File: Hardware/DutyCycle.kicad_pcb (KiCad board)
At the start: 2 copper layers, 40 x 20 mm, 39 parts, among them J1 LiPo, J2 USB, J4 MOT, Q1 AO3400A, Q2 AO3400A, Q3 AO3401A, SW1 SW_Push, U1 AT32F421KxU7, U3 ME6211C28M5, U5 TP4055

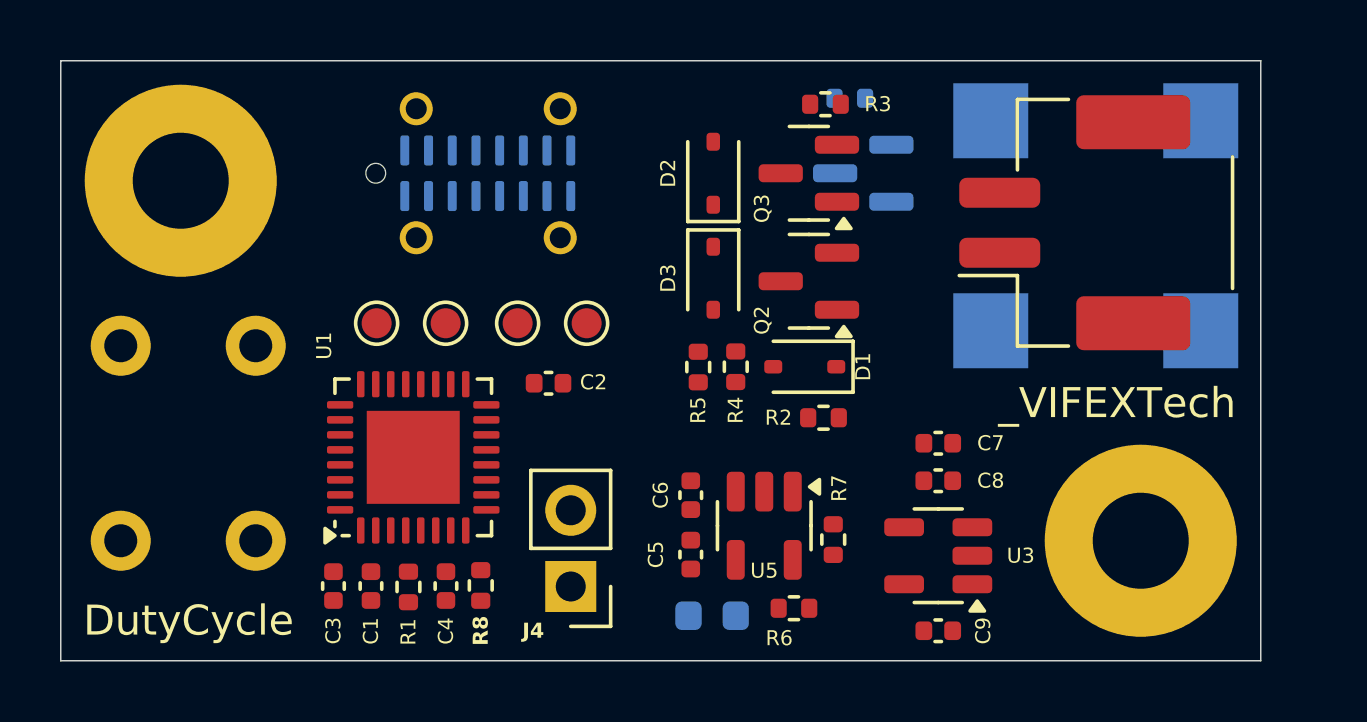
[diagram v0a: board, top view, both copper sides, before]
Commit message: feat(pcb): finish PCB layout
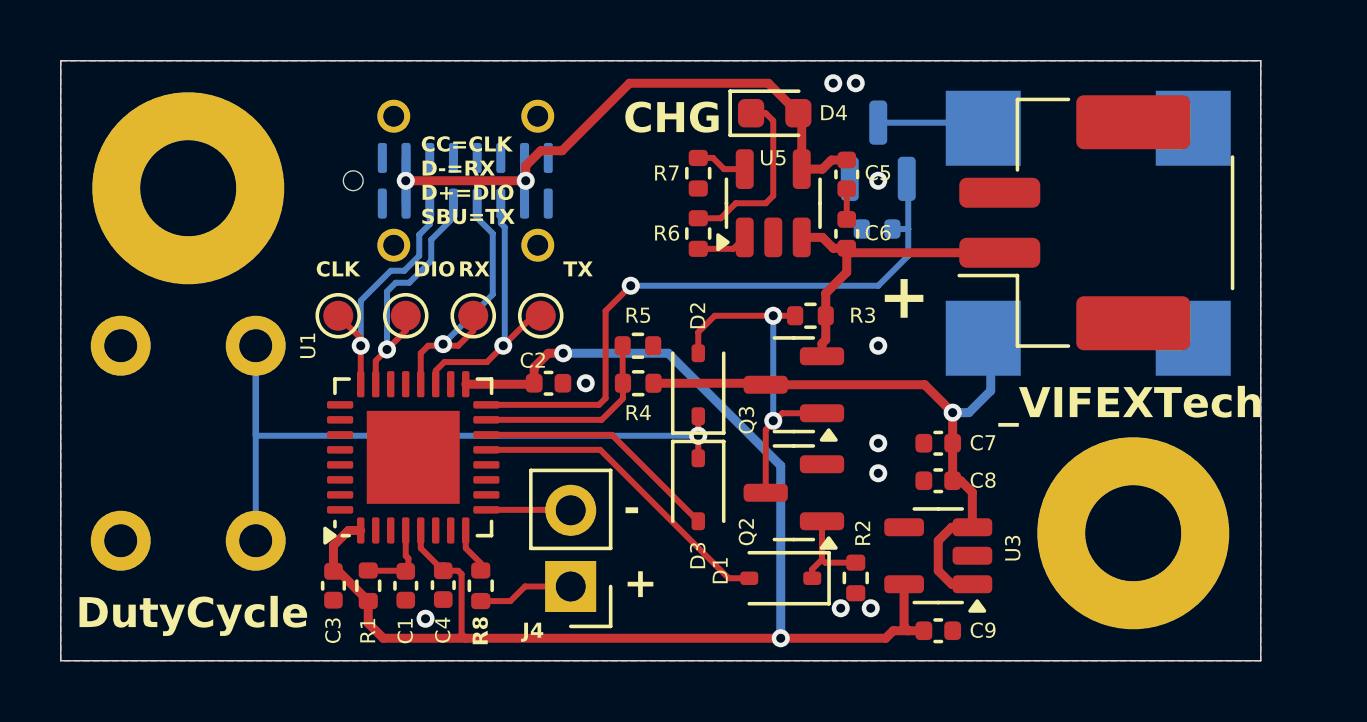
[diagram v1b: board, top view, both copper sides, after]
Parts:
- D4: moved to F.Cu
- moved D4 16.9 mm to (98.8, 76.8), turned to 0 degrees
- moved C5 13.7 mm to (101.2, 78.8), turned to -90 degrees
- moved R7 13.0 mm to (96.2, 78.8), turned to 90 degrees
- moved R6 12.9 mm to (96.2, 80.8), turned to 90 degrees
- moved U5 10.8 mm to (98.8, 79.8), turned to 90 degrees
- moved C6 10.1 mm to (101.2, 80.8), turned to 90 degrees
- moved D1 7.10 mm to (99.0, 92.2)
- moved Q2 7.07 mm to (99.4, 89.4)
- moved D2 7.07 mm to (96.2, 85.8)
- moved D3 7.07 mm to (96.2, 89.3)
- moved Q3 7.07 mm to (99.4, 85.8)
- moved R3 7.07 mm to (100.0, 83.5)
- moved R2 5.45 mm to (101.5, 92.2), turned to -90 degrees
- moved R9 4.45 mm to (102.2, 80.6)
- moved TP3 3.74 mm to (86.5, 83.5)
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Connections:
- J2 pad A5: /DEBUG_TX -> /SWCLK
- J2 pad A6: /DEBUG_RX -> /SWDIO
- J2 pad A7: /SWDIO -> /DEBUG_RX
- J2 pad A8: /SWCLK -> /DEBUG_TX
- J2 pad B5: /DEBUG_TX -> unconnected-(J2-CC2-PadB5)
- J2 pad B6: /DEBUG_RX -> unconnected-(J2-D+-PadB6)
- J2 pad B7: /SWDIO -> unconnected-(J2-D--PadB7)
- J2 pad B8: /SWCLK -> unconnected-(J2-SBU2-PadB8)
- U1 pad 13: unconnected-(U1-PA7-Pad13) -> /PWR_EN
- U1 pad 14: /MOT_OUT1 -> /KEY_DET
- U1 pad 15: /MOT_OUT2 -> /BAT_DET
- U1 pad 16: unconnected-(U1-PB2-Pad16) -> /BUZZ
- U1 pad 25: /PWR_EN -> unconnected-(U1-PA15-Pad25)
- U1 pad 26: /KEY_DET -> unconnected-(U1-PB3-Pad26)
- U1 pad 6: /BAT_DET -> unconnected-(U1-PA0-Pad6)
- U1 pad 7: /BUZZ -> unconnected-(U1-PA1-Pad7)
- U1 pad 8: unconnected-(U1-PA2-Pad8) -> /MOT_OUT1
- U1 pad 9: unconnected-(U1-PA3-Pad9) -> /MOT_OUT2
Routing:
- net VDD: track 0.00 -> 47.9 mm, vias 0 -> 2
- net Net-(D2-K): track 0.00 -> 25.7 mm, vias 0 -> 1
- net VBAT: track 0.00 -> 21.8 mm, vias 0 -> 1
- net VBUS: track 0.00 -> 21.8 mm, vias 0 -> 2
- net /BUZZ: track 0.00 -> 21.0 mm, vias 0 -> 1
- net Net-(D2-A): track 0.00 -> 11.9 mm, vias 0 -> 2
- net /BAT_IN: track 0.00 -> 10.8 mm
- net /PWR_EN: track 0.00 -> 10.5 mm
- net /DEBUG_RX: track 0.00 -> 9.94 mm, vias 0 -> 1
- net /SWCLK: track 0.00 -> 9.61 mm, vias 0 -> 1
- net /DEBUG_TX: track 0.00 -> 9.52 mm, vias 0 -> 1
- net /SWDIO: track 0.00 -> 8.80 mm, vias 0 -> 1
- net /KEY_DET: track 0.00 -> 8.26 mm
- net /BAT_DET: track 0.00 -> 6.61 mm
- net Net-(D4-K): track 0.00 -> 6.15 mm
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- added copper zone on B.Cu, net GND
- added copper zone on F.Cu, net GND
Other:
- board text added: "${TITLE}"
- board text added: "+"
- board text added: "-"
- board text added: "CC=CLK D-=RX D+=DIO SBU=TX"
- board text added: "CHG"
- board text added: "CLK"
- board text added: "DIO"
- board text added: "REV: ${REVISION} ${CURRENT_DATE}"
- board text added: "RX"
- board text added: "TX"
- board text removed: "DutyCycle"
